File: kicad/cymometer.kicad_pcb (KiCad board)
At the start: 2 copper layers, 190.9 x 62.4 mm, 62 parts, among them IC1 ATMEGA8-P, P1 BNC, P2 CONN_2, P3 CONN_3X2, P4 CONN_7, P5 CONN_7, P6 CONN_12, P7 CONN_12, Q1 BC550, SW1 switch_3, U1 7805, X1 20.48 MГц

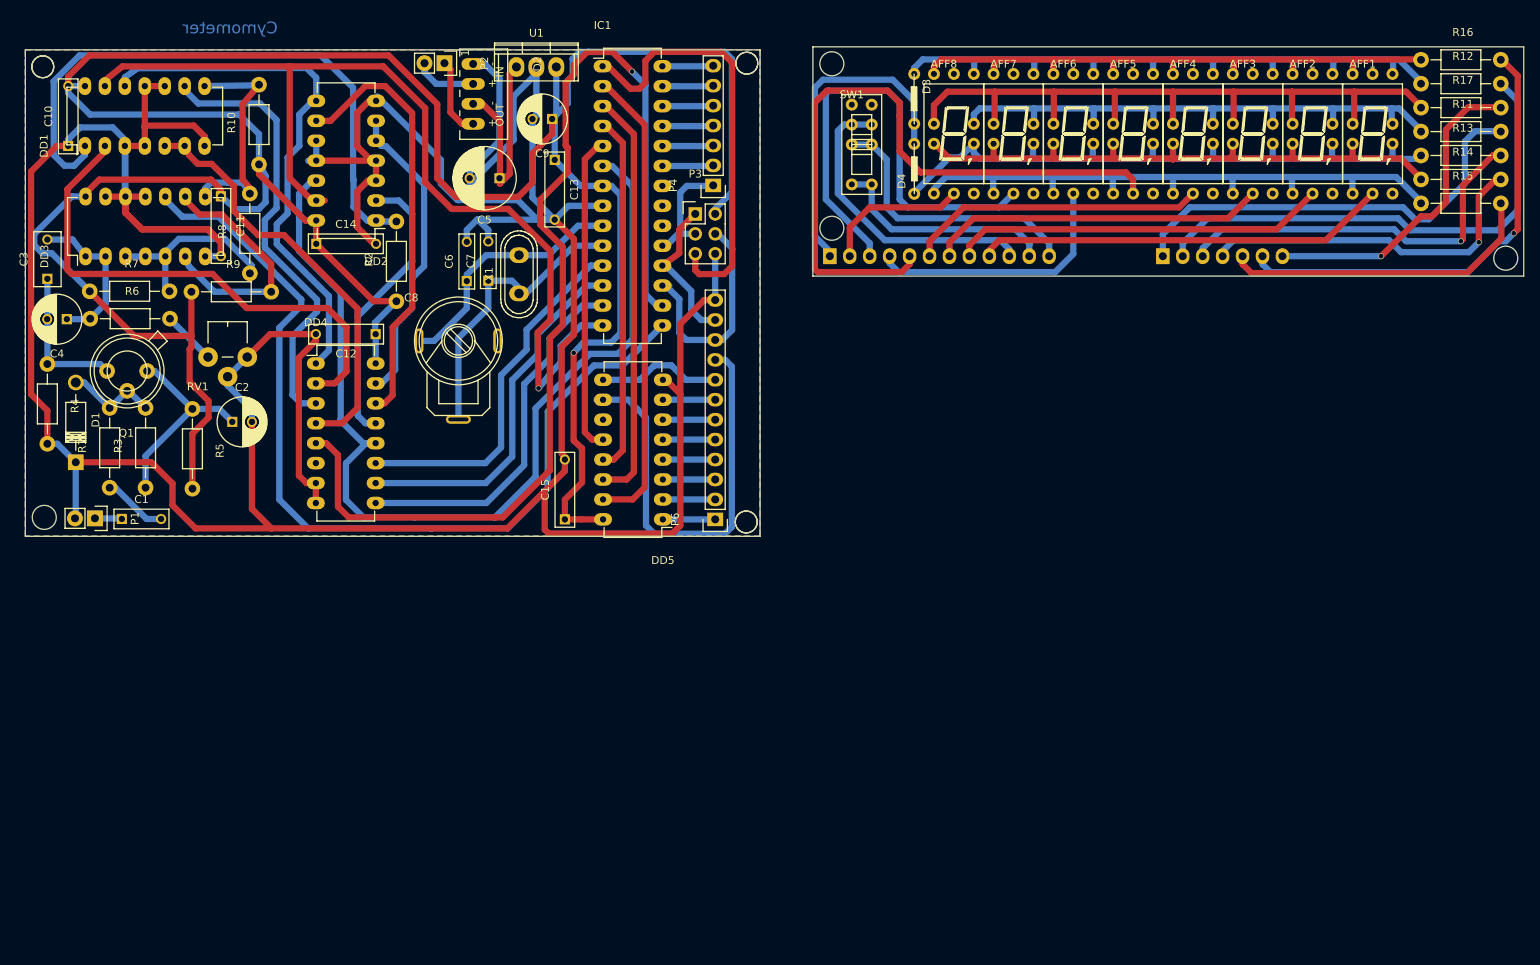
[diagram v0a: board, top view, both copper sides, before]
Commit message: Add size
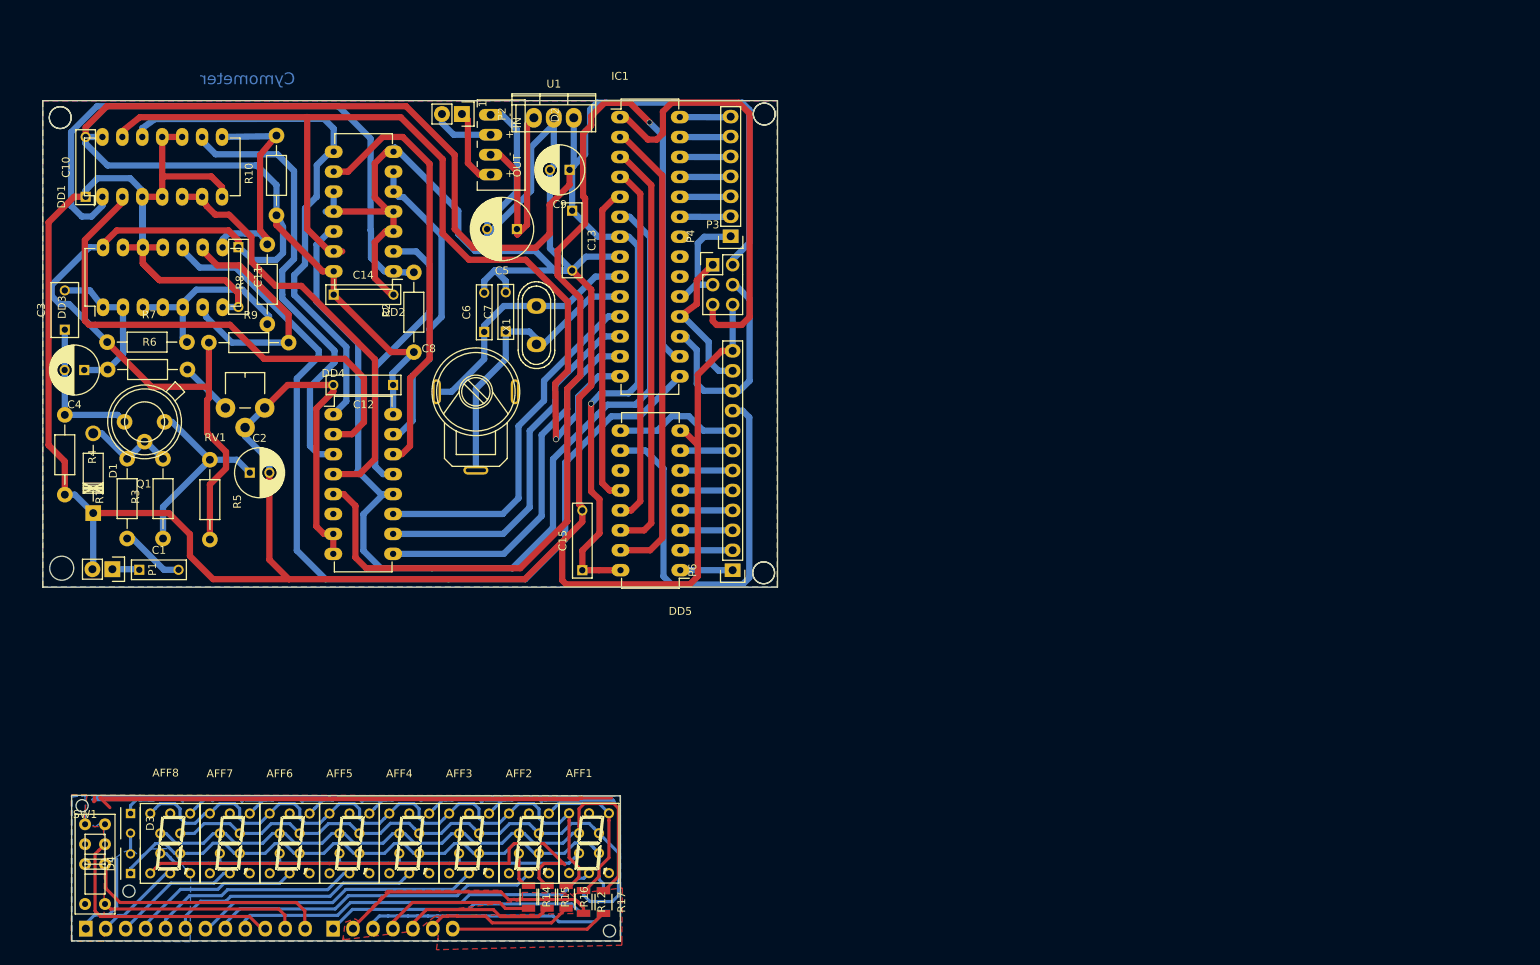
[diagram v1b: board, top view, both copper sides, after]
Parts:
- AFF1, AFF2, AFF3, AFF4, AFF5, AFF6, AFF7, AFF8: footprint cymometer:7segment_small -> cymometer:7segment_small1
- D3, D4: footprint cymometer:LED -> Capacitors_ThroughHole:C_Rect_L4_W2.5_P2.5
- R11, R13: footprint Resistors_ThroughHole:Resistor_Horizontal_RM10mm -> Resistors_SMD:R_1206; moved to B.Cu
- R12, R14, R15, R16, R17: footprint Resistors_ThroughHole:Resistor_Horizontal_RM10mm -> Resistors_SMD:R_1206
- moved R16 152.4 mm to (97.7, 126.1), turned to 270 degrees
- moved R12 149.2 mm to (99.9, 126.7), turned to 270 degrees
- moved R14 145.9 mm to (92.9, 126.1), turned to 270 degrees
- moved R17 145.2 mm to (102.5, 126.7), turned to 270 degrees
- moved R11 145.0 mm to (99.9, 126.7), turned to 270 degrees
- moved R15 142.1 mm to (95.3, 126.1), turned to 270 degrees
- moved R13 141.0 mm to (102.5, 126.7), turned to 270 degrees
- moved P5 136.1 mm to (68.0, 130.1)
- moved AFF4 134.7 mm to (77.7, 119.3)
- moved AFF5 134.7 mm to (70.1, 119.3)
- moved AFF6 134.7 mm to (62.5, 119.3)
- moved AFF7 134.7 mm to (54.9, 119.3)
- moved AFF8 134.7 mm to (47.3, 119.3)
- moved D3 134.7 mm to (42.2, 115.4)
- moved D4 134.7 mm to (42.2, 123.1)
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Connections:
- AFF1 pad 5: (no net) -> Net-(AFF1-Pad5)
- AFF1 pad 8: (no net) -> Net-(AFF1-Pad8)
- AFF2 pad 5: (no net) -> Net-(AFF2-Pad5)
- AFF2 pad 8: (no net) -> Net-(AFF2-Pad8)
- AFF3 pad 5: (no net) -> Net-(AFF3-Pad5)
- AFF3 pad 8: (no net) -> Net-(AFF3-Pad8)
- AFF4 pad 5: (no net) -> Net-(AFF4-Pad5)
- AFF4 pad 8: (no net) -> Net-(AFF4-Pad8)
- AFF5 pad 5: (no net) -> Net-(AFF5-Pad5)
- AFF5 pad 8: (no net) -> Net-(AFF5-Pad8)
- AFF6 pad 5: (no net) -> Net-(AFF6-Pad5)
- AFF6 pad 8: (no net) -> Net-(AFF6-Pad8)
- AFF7 pad 5: (no net) -> Net-(AFF7-Pad5)
- AFF7 pad 8: (no net) -> Net-(AFF7-Pad8)
- AFF8 pad 5: (no net) -> Net-(AFF8-Pad5)
- AFF8 pad 8: (no net) -> Net-(AFF8-Pad8)
- DD3 pad 11: (no net) -> GND
- DD3 pad 12: (no net) -> GND
- DD3 pad 13: (no net) -> GND
- DD4 pad 6: (no net) -> Net-(DD4-Pad6)
- DD5 pad 11: (no net) -> Net-(DD5-Pad11)
- IC1 pad 20: (no net) -> Net-(IC1-Pad20)
- IC1 pad 21: (no net) -> Net-(IC1-Pad21)
- IC1 pad 22: (no net) -> Net-(IC1-Pad22)
- SW1 pad 4: (no net) -> Net-(SW1-Pad4)
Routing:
- net (no net): track 0.00 -> 128.6 mm
- net Net-(AFF1-Pad6): track 82.3 -> 182.8 mm
- net Net-(AFF5-Pad3): track 86.2 -> 27.7 mm
- net Net-(AFF7-Pad3): track 61.2 -> 16.2 mm
- net Net-(P5-Pad6): track 58.7 -> 18.9 mm, vias 1 -> 0
- net Net-(P5-Pad2): track 64.4 -> 32.8 mm
- net Net-(D3-Pad2): track 42.0 -> 14.3 mm
- net Net-(P5-Pad4): track 43.8 -> 19.6 mm, vias 1 -> 0
- net Net-(P5-Pad1): track 55.7 -> 33.8 mm
- net Net-(P5-Pad5): track 40.8 -> 19.3 mm
- net Net-(P5-Pad7): track 41.2 -> 20.2 mm, vias 1 -> 0
- net Net-(P5-Pad3): track 49.3 -> 31.2 mm, vias 1 -> 0
- net Net-(AFF1-Pad1): track 79.7 -> 63.4 mm
- net Net-(AFF1-Pad10): track 95.0 -> 80.5 mm
- net Net-(AFF1-Pad2): track 80.1 -> 66.9 mm
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- added copper zone on F.Cu, net Net-(AFF1-Pad1)
- added copper zone on B.Cu, net Net-(AFF1-Pad6)
- added copper zone on B.Cu, net Net-(D3-Pad2)
- added copper zone on F.Cu, net Net-(P5-Pad2)
- added copper zone on B.Cu, net Net-(P5-Pad3)
- added copper zone on F.Cu, net Net-(P5-Pad7)
- added copper zone on F.Cu, net Net-(P7-Pad10)
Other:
- board size 190.9 x 62.4 mm -> 93.6 x 107 mm
- net class Default: clearance 0.6 -> 0.3; trace_width 0.8 -> 0.4
- rule trace_clearance: 0.6 -> 0.3
- rule trace_min: 0.7 -> 0.2
